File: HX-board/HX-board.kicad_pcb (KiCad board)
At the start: 2 copper layers, 63.5 x 63.5 mm, 101 parts, among them J1 Testpoints, J2 PCIE-LP-01-01-F-DV-A-TR, J3 DB15_Female, J4 Testpoints, J5 DB15_Female, Q1 MMBT4403LT3G, Q2 MMBT4403LT3G, Q3 MMBT4403LT3G, Q4 MMBT4403LT3G, Q5 MMBT4403LT3G, Q6 MMBT4403LT3G, Q7 MMBT4403LT3G, Q8 MMBT4403LT3G, U1 HX711, U2 HX711, U3 HX711, U4 HX711, U5 HX711, U6 HX711, U7 HX711, U8 HX711

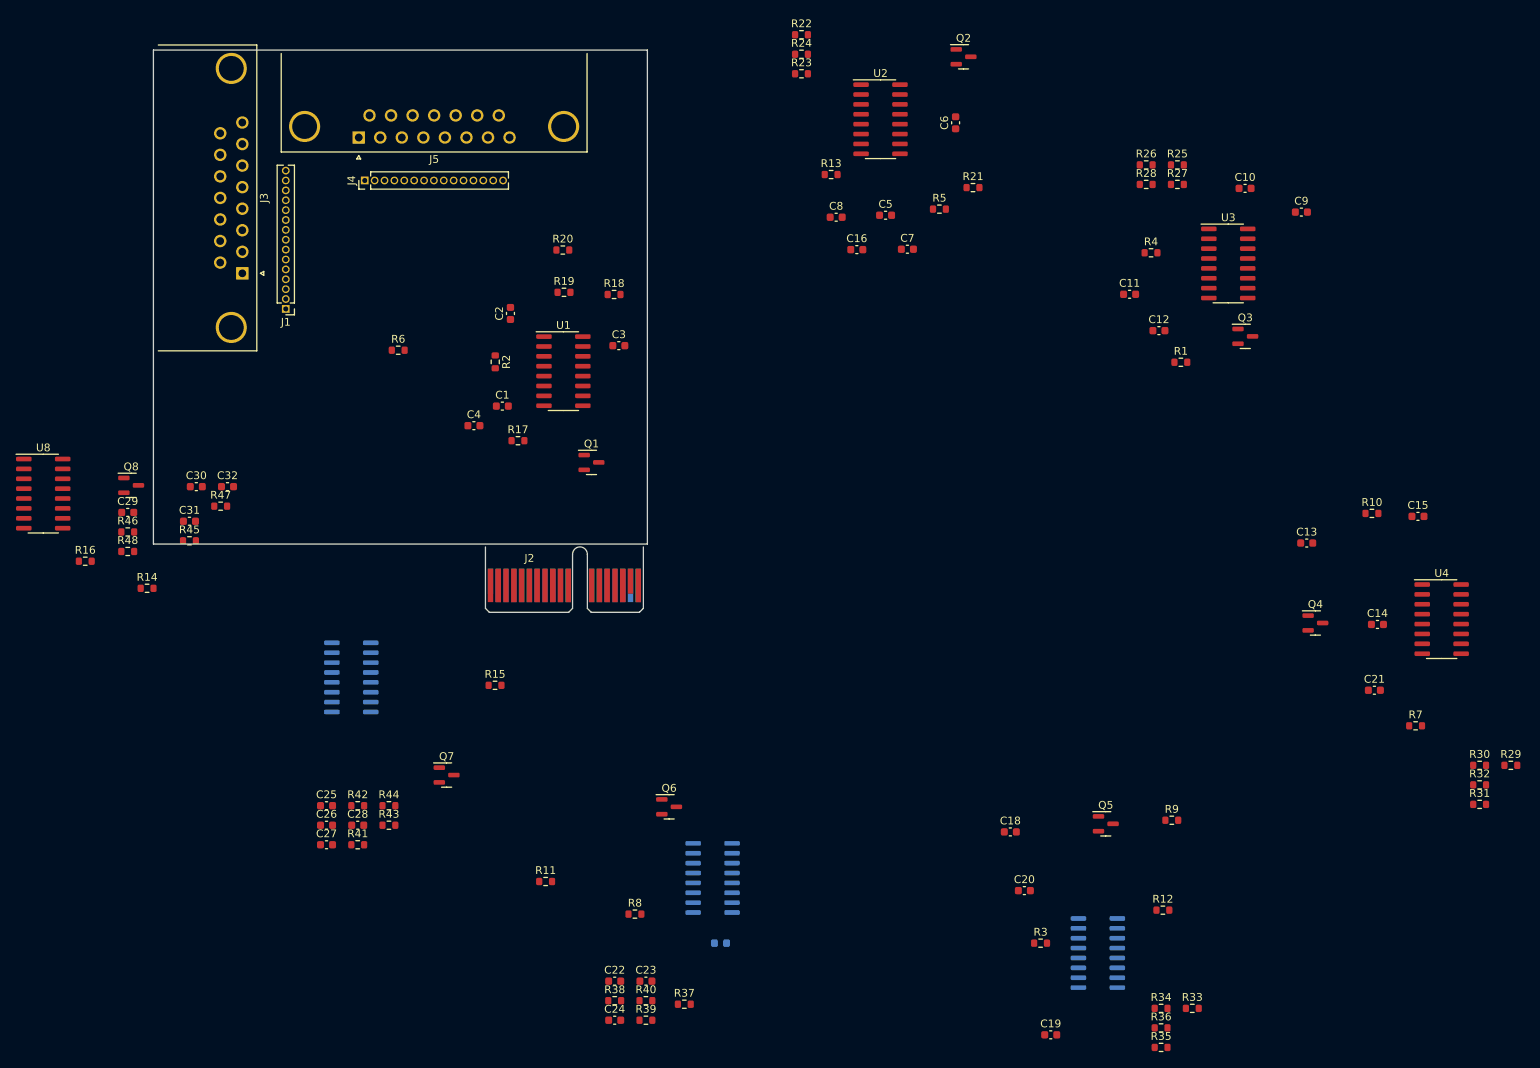
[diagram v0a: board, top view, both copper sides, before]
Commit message: Revert "Revert "HX and TC Board mostly finished""
This reverts commit 2ae13608b6027366e1c59111a8dca91d16e06deb.
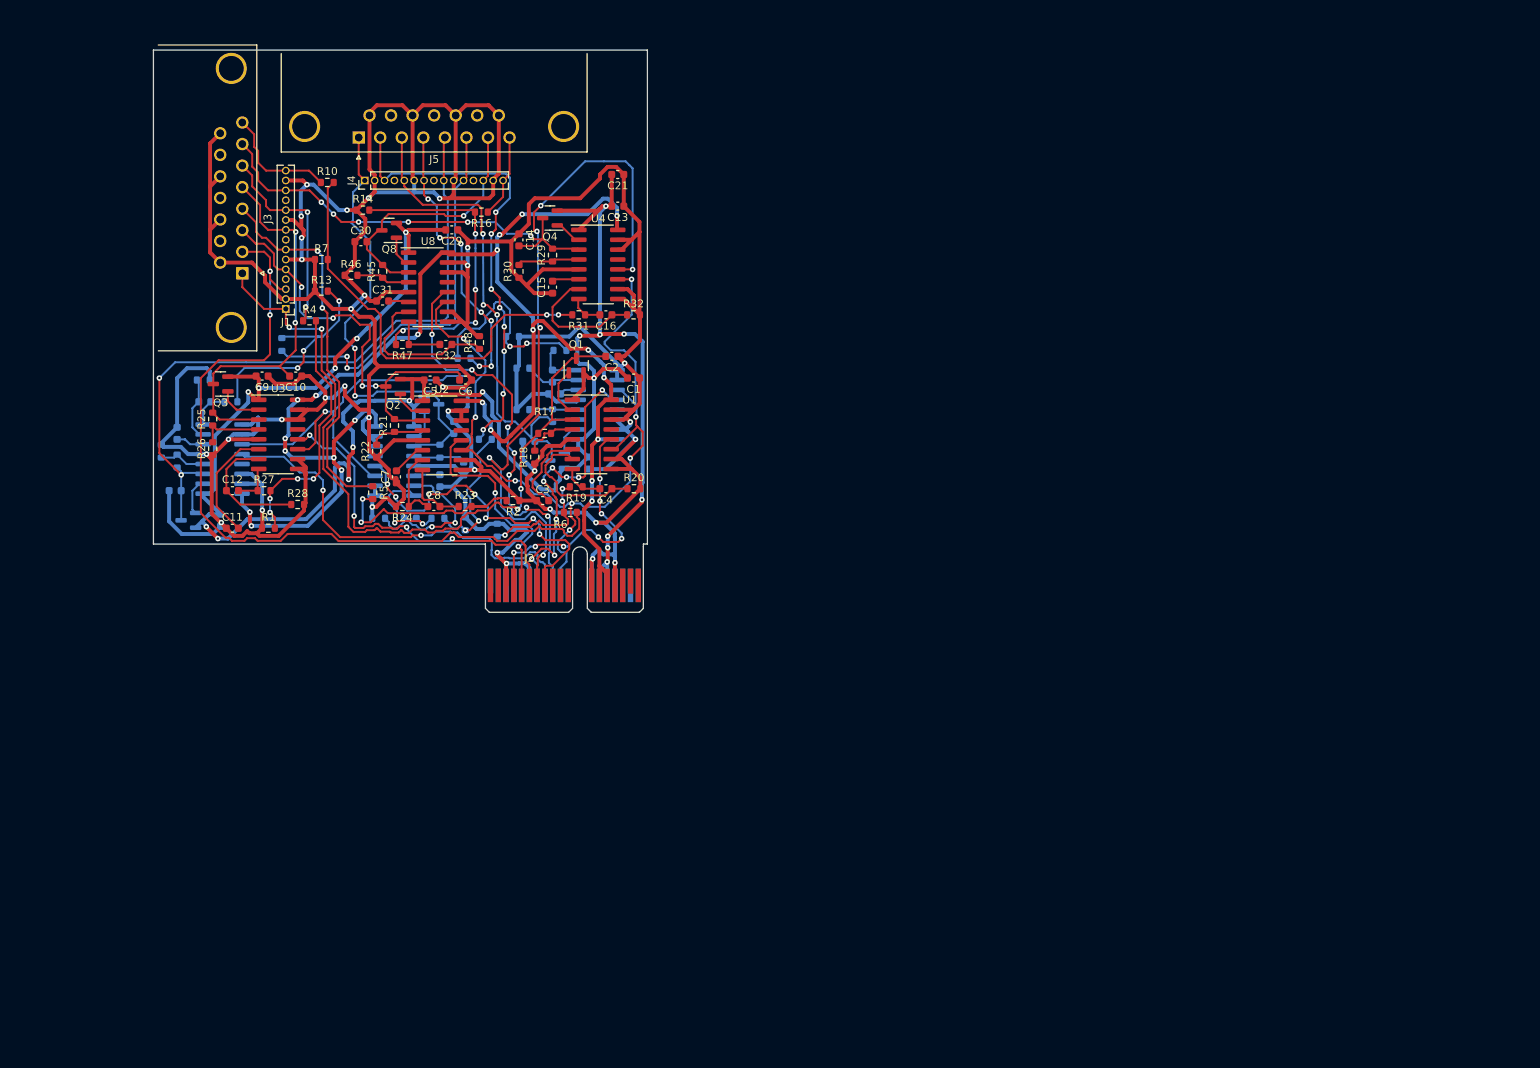
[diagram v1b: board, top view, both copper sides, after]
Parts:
- C18, C19, C20, C22, C23, C24, C25, C26, C27, C28, Q5, Q6, Q7, R11, R12, R15, R3, R33, R34, R35, R36, R37, R38, R39, R40, R41, R42, R43, R44, R8, R9: moved to B.Cu
- moved R7 152.9 mm to (123.2, 90.4)
- moved R10 140.9 mm to (124.0, 80.5)
- moved R29 139.6 mm to (152.9, 89.9), turned to 90 degrees
- moved R30 138.9 mm to (148.6, 91.9), turned to 90 degrees
- moved C9 135.3 mm to (115.6, 105.4), turned to 180 degrees
- moved Q3 131.9 mm to (110.2, 106.4), turned to 180 degrees
- moved R31 131.8 mm to (156.3, 97.5), turned to 180 degrees
- moved R25 128.2 mm to (109.2, 110.9), turned to 90 degrees
- moved R26 125.4 mm to (109.2, 114.7), turned to 90 degrees
- moved R32 124.4 mm to (163.3, 97.5)
- moved C10 124.4 mm to (119.9, 105.4), turned to 180 degrees
- moved U3 124.1 mm to (117.6, 112.9)
- moved R27 123.8 mm to (115.8, 120.1)
- moved C14 120.9 mm to (148.6, 87.9), turned to -90 degrees
- moved C12 120.9 mm to (111.8, 120.1)
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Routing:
- net GND: track 0.00 -> 697.2 mm, vias 0 -> 33
- net +5V: track 0.00 -> 273.3 mm, vias 0 -> 20
- net +3.3V: track 0.00 -> 194.6 mm, vias 0 -> 22
- net /HX_CLK: track 0.00 -> 157.9 mm, vias 0 -> 9
- net /HX1_A+: track 0.00 -> 104.5 mm, vias 0 -> 2
- net /HX1_E+: track 0.00 -> 98.3 mm, vias 0 -> 4
- net /HX4_DT: track 0.00 -> 92.0 mm, vias 0 -> 6
- net /HX7_E+: track 0.00 -> 87.2 mm, vias 0 -> 2
- net /HX6_E+: track 0.00 -> 64.8 mm, vias 0 -> 3
- net /HX5_A+: track 0.00 -> 59.8 mm, vias 0 -> 8
- net /HX5_E+: track 0.00 -> 59.5 mm, vias 0 -> 2
- net /HX4_E+: track 0.00 -> 56.5 mm, vias 0 -> 6
- net /HX2_E+: track 0.00 -> 56.0 mm, vias 0 -> 4
- net /HX711 4/A+: track 0.00 -> 54.4 mm, vias 0 -> 2
- net /HX7_DT: track 0.00 -> 53.2 mm, vias 0 -> 2
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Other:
- board size 63.5 x 63.5 mm -> 63.5 x 63.9 mm

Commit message: Revert "HX and TC Board mostly finished"
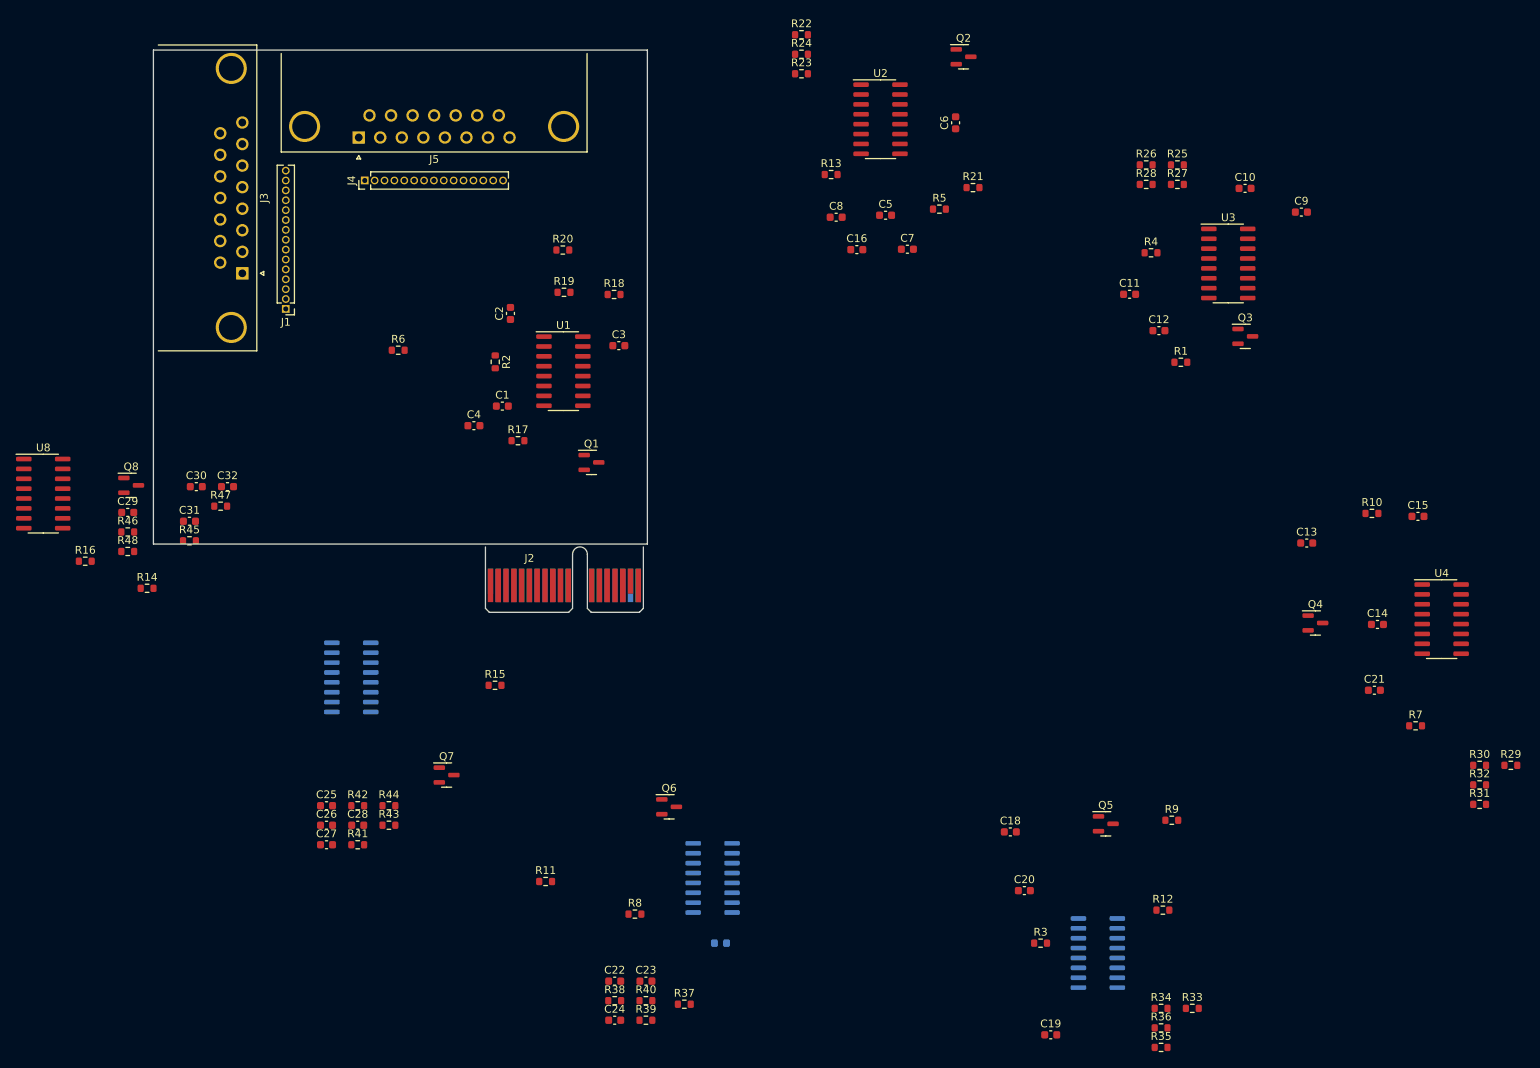
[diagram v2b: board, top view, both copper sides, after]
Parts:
- C18, C19, C20, C22, C23, C24, C25, C26, C27, C28, Q5, Q6, Q7, R11, R12, R15, R3, R33, R34, R35, R36, R37, R38, R39, R40, R41, R42, R43, R44, R8, R9: moved to F.Cu
- moved R7 152.9 mm to (263.9, 150.4)
- moved R10 140.9 mm to (258.2, 123.1)
- moved R29 139.6 mm to (276.1, 155.4), turned to 0 degrees
- moved R30 138.9 mm to (272.1, 155.4), turned to 0 degrees
- moved C9 135.3 mm to (249.2, 84.3), turned to 0 degrees
- moved Q3 131.9 mm to (242.0, 100.3), turned to 0 degrees
- moved R31 131.8 mm to (272.1, 160.5), turned to 0 degrees
- moved R25 128.2 mm to (233.2, 78.3), turned to 0 degrees
- moved R26 125.4 mm to (229.2, 78.3), turned to 0 degrees
- moved R32 124.4 mm to (272.1, 158.0)
- moved C10 124.4 mm to (241.9, 81.3), turned to 0 degrees
- moved U3 124.1 mm to (239.8, 90.9)
- moved R27 123.8 mm to (233.2, 80.8)
- moved C14 120.9 mm to (259.0, 137.3), turned to 0 degrees
- moved C12 120.9 mm to (230.9, 99.6)
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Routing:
- net GND: track 697.2 -> 0.00 mm, vias 33 -> 0
- net +5V: track 273.3 -> 0.00 mm, vias 20 -> 0
- net +3.3V: track 194.6 -> 0.00 mm, vias 22 -> 0
- net /HX_CLK: track 157.9 -> 0.00 mm, vias 9 -> 0
- net /HX1_A+: track 104.5 -> 0.00 mm, vias 2 -> 0
- net /HX1_E+: track 98.3 -> 0.00 mm, vias 4 -> 0
- net /HX4_DT: track 92.0 -> 0.00 mm, vias 6 -> 0
- net /HX7_E+: track 87.2 -> 0.00 mm, vias 2 -> 0
- net /HX6_E+: track 64.8 -> 0.00 mm, vias 3 -> 0
- net /HX5_A+: track 59.8 -> 0.00 mm, vias 8 -> 0
- net /HX5_E+: track 59.5 -> 0.00 mm, vias 2 -> 0
- net /HX4_E+: track 56.5 -> 0.00 mm, vias 6 -> 0
- net /HX2_E+: track 56.0 -> 0.00 mm, vias 4 -> 0
- net /HX711 4/A+: track 54.4 -> 0.00 mm, vias 2 -> 0
- net /HX7_DT: track 53.2 -> 0.00 mm, vias 2 -> 0
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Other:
- board size 63.5 x 63.9 mm -> 63.5 x 63.5 mm
